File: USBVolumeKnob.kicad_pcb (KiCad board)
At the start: 4 copper layers, 65.6 x 66 mm, 74 parts, among them J1 Conn_01x04, J2 Conn_01x09, J3 USB_C_Receptacle_USB2.0, J4 FTSH-105-01, SW1 SW_Push, SW2 SW_Push, SW3 SW_Push, SW4 SW_Push, U1 PEC12R-4xxxF, U2 LT1963AxST-3.3, U3 SN74LV1T125, U4 SN74LV1T125, U5 STM32F401RCTx, U6 USBLC6-2SC6, Y1 X1G004451000200

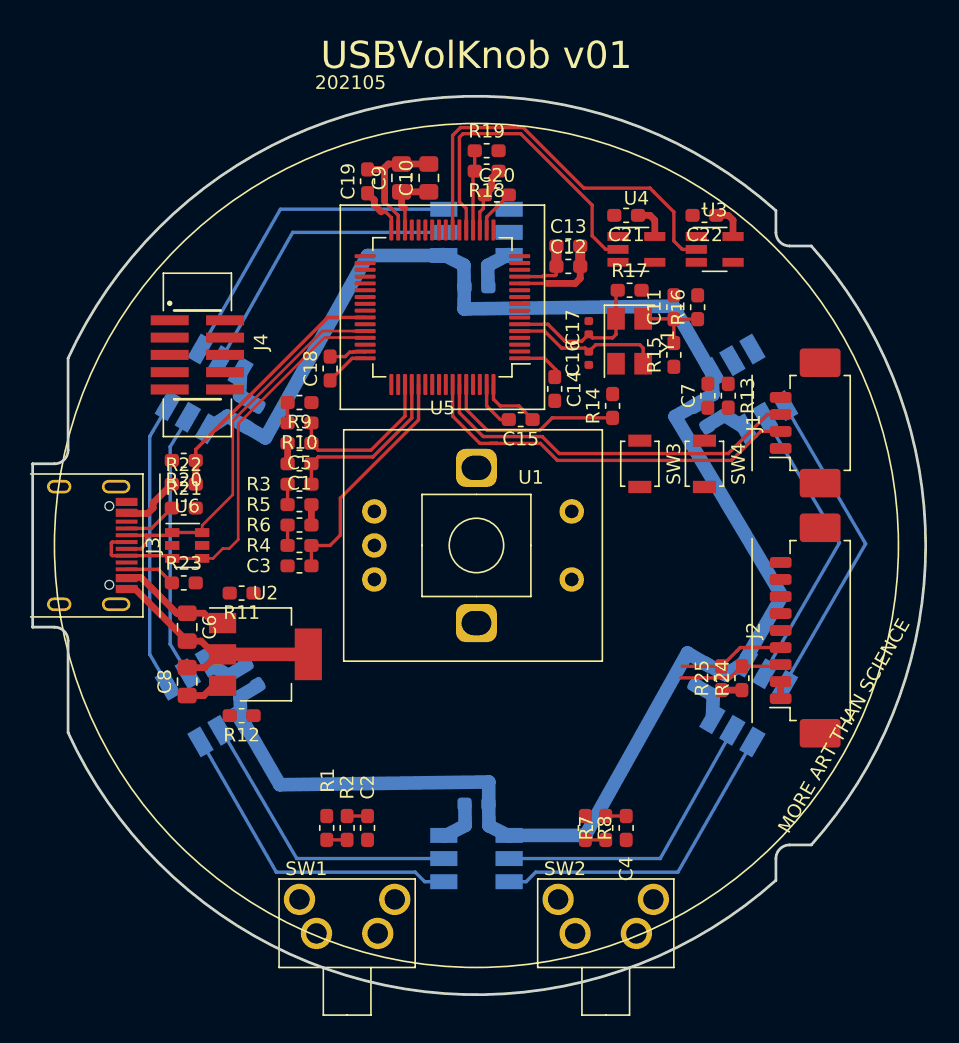
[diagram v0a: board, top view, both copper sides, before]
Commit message: Completed v02. Final schematic and layout.
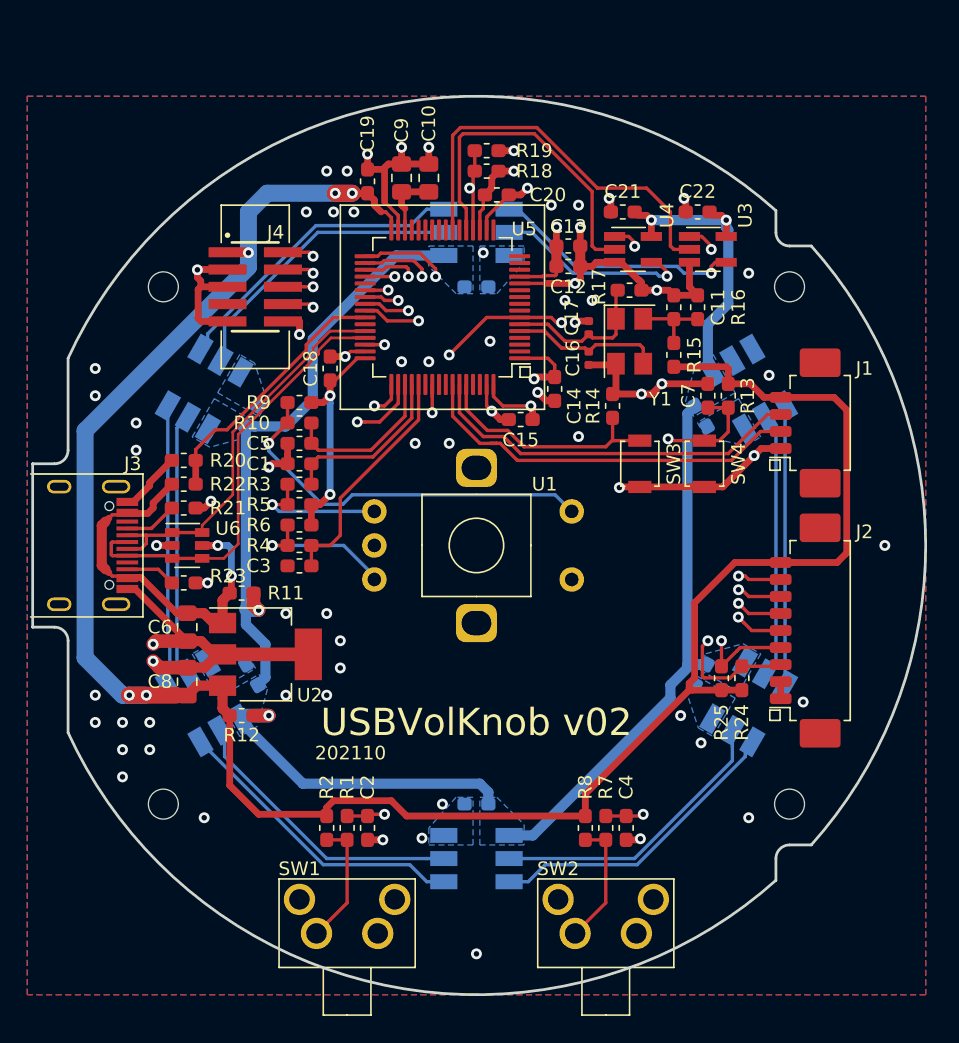
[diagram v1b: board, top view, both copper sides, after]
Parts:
- added M1: MountingHole_2.2mm_M2_ISO14580, MountingHole:MountingHole_2.2mm_M2_ISO14580, F.Cu at (129.0, 83.0)
- added M2: MountingHole_2.2mm_M2_ISO14580, MountingHole:MountingHole_2.2mm_M2_ISO14580, F.Cu at (175.0, 83.0)
- added M3: MountingHole_2.2mm_M2_ISO14580, MountingHole:MountingHole_2.2mm_M2_ISO14580, F.Cu at (175.0, 121.0)
- added M4: MountingHole_2.2mm_M2_ISO14580, MountingHole:MountingHole_2.2mm_M2_ISO14580, F.Cu at (129.0, 121.0)
- moved J4 6.56 mm to (135.8, 83.0)
- moved C22 0.56 mm to (168.2, 77.5)
- moved U3 0.50 mm to (169.0, 80.2)
- moved C21 0.35 mm to (162.8, 77.5)
- moved U4 0.25 mm to (163.5, 80.2)
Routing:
- net +3V3: track 30.8 -> 203.6 mm, vias 0 -> 11
- net GND: track 66.9 -> 125.2 mm, vias 0 -> 71
- net /BTN1: track 1.50 -> 58.0 mm, vias 0 -> 2
- net /BTN0: track 1.50 -> 57.5 mm, vias 0 -> 2
- net /NRST: track 0.00 -> 52.5 mm, vias 0 -> 4
- net /PB14: track 0.00 -> 44.8 mm, vias 0 -> 2
- net /PB15: track 0.00 -> 44.8 mm, vias 0 -> 2
- net /PB13: track 0.00 -> 44.3 mm, vias 0 -> 2
- net /PB12: track 0.00 -> 43.2 mm, vias 0 -> 2
- net /PC09: track 7.75 -> 49.4 mm, vias 0 -> 2
- net /PA08: track 7.79 -> 47.3 mm, vias 0 -> 2
- net Net-(R10-Pad2): track 1.50 -> 28.8 mm, vias 0 -> 1
- net /SPI_EN: track 5.88 -> 30.3 mm, vias 0 -> 3
- net /SWO: track 0.00 -> 20.4 mm, vias 0 -> 2
- net /MOSI_5V0: track 0.00 -> 18.5 mm, vias 0 -> 1
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- added copper zone on In1.Cu, net +3V3
- added copper zone on B.Cu, net GND
- added copper zone on F.Cu, net GND
- added copper zone on In1.Cu, net GND
- added copper zone on In2.Cu, net GND
- added copper zone on B.Cu, net VDD
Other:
- board text added: "202110"
- board text added: "FAB NOTES: 1. FABRICATE PCB IN ACCORDANCE WITH THE CURRENT REVISION OF IPC-6012, CLASS 2. 2. MATERIAL SHALL BE FR4 Tg 180 C OR EQUIVALENT. 3. MATERIAL SHALL BE RoHS COMPLIANT, LEAD FREE, HALOGEN FREE. 4. ENIG PLATING PER CURRENT REVISION OF IPC-4552. 5. PLATING IN HOLES SHALL BE CONTINUOUS ELECTROLYTIC COPPER WITH 0.025 MM MINIMUM BARREL THICKNESS. FINISHED HOLE SIZE MEASURED AFTER PLATING. 6. SO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"
- board text added: "USBVolKnob v02"
- board text removed: "202105"
- board text removed: "USBVolKnob v01"
